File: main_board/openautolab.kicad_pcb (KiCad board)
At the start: 2 copper layers, 98 x 84 mm, 64 parts, among them J1 GP7, J10 FILTER_PUMP, J11 FILTER_SENSOR, J12 PWR_IN, J13 HX711, J14 SERVO, J15 Display, J2 GP6, J3 GP5, J4 GP4, J5 GP3, J6 GP2, J7 GP1, J8 GP0, J9 PUMP, Q1 TSM2302CX, Q2 TSM2302CX, Q3 TSM2302CX, Q4 TSM2302CX, Q5 TSM2302CX, Q6 TSM2302CX, Q7 TSM2302CX, Q8 TSM2302CX, Q9 TSM2302CX, SW0 GP20, SW1 GP21, SW2 GP22, SW3 SW_DPST_x2, U2 LM2575-5.0BT, U3 Pico, U4 A4950E

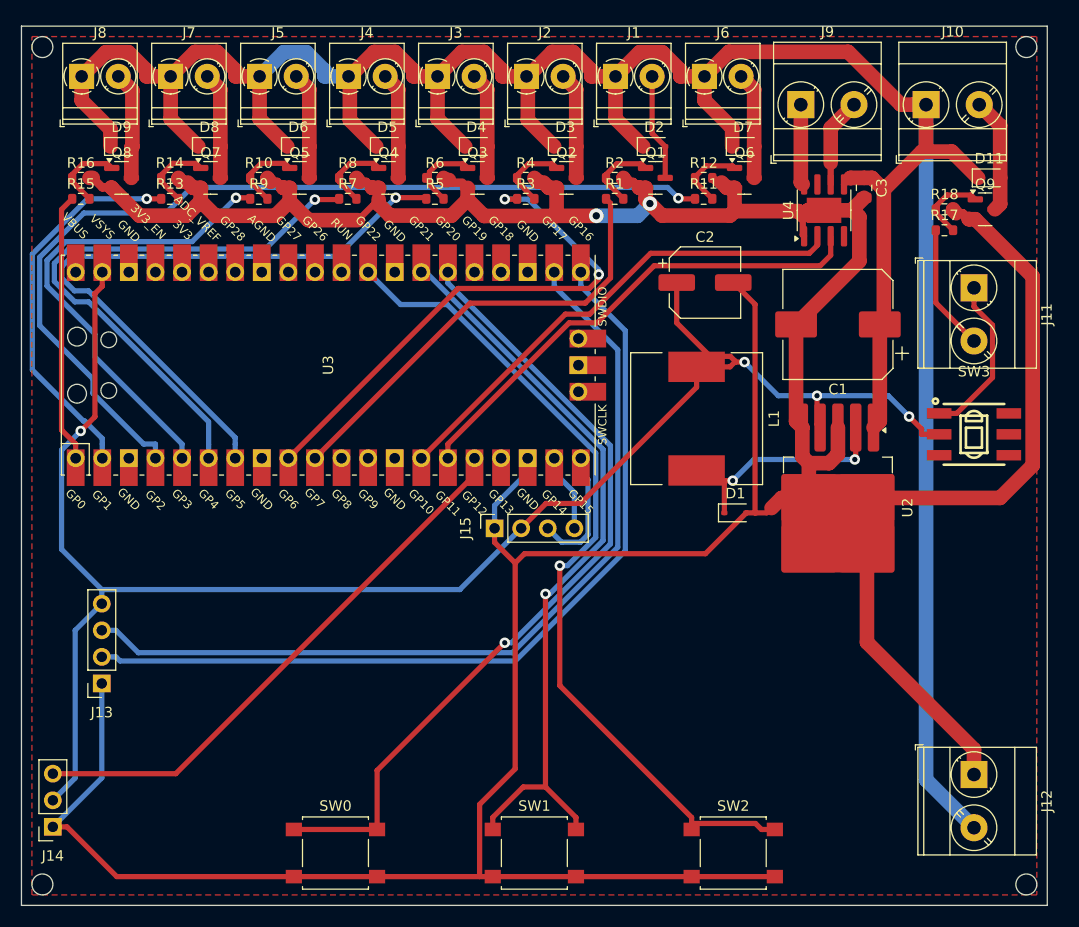
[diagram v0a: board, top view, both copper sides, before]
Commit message: minor routing-related stuff
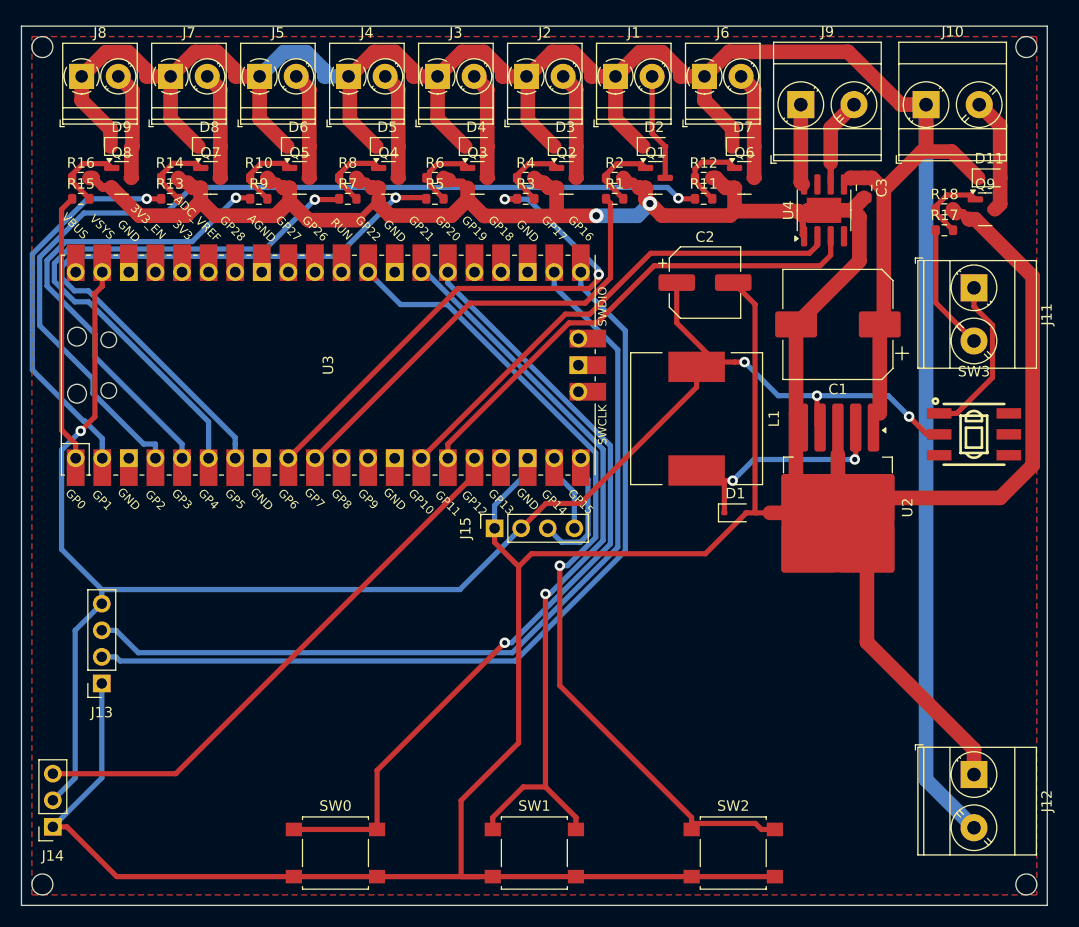
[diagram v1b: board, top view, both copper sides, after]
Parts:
- SW3: footprint easyeda2kicad:SW-SMD_6P-L5.8-W5.8-P2.00-LS8.0_YTSPS-22E58LM -> JLCPCB:SW-SMD_6P-L5.8-W5.8-P2.00-LS8.0_YTSPS-22E58LM
- U3: footprint RP-Pico:RPi_Pico_SMD_TH -> RPi Pico:RPi_Pico_SMD_TH
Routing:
- net +5V: track 163.1 -> 158.9 mm
- net GNDPWR: track 242.2 -> 246.3 mm
- net GND: track 178.0 -> 180.5 mm
- net +12V: track 276.5 -> 274.9 mm
- net Net-(Q6-G): track 7.06 -> 7.81 mm
